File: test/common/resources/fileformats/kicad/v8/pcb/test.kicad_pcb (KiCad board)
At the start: 2 copper layers, 4 parts

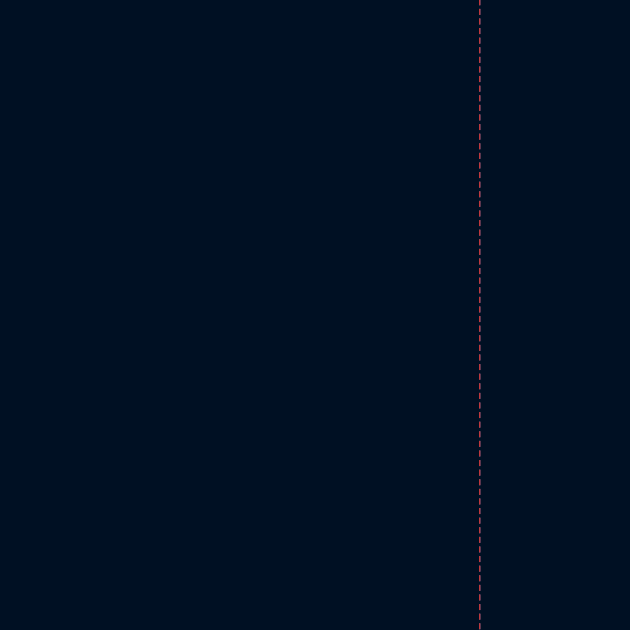
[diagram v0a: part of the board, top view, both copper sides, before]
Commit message: reset test file
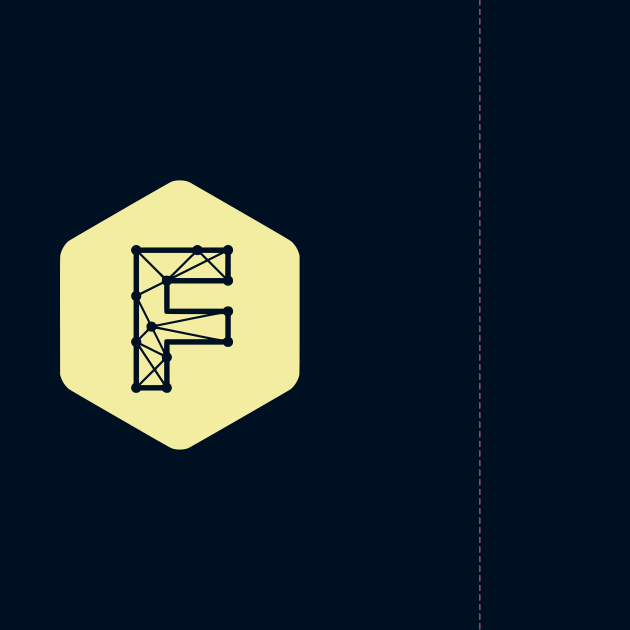
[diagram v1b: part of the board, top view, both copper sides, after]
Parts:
- G***: moved to F.Cu
- moved G*** 22.4 mm to (10.0, 20.0), turned to 0 degrees

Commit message: fast without cacheing
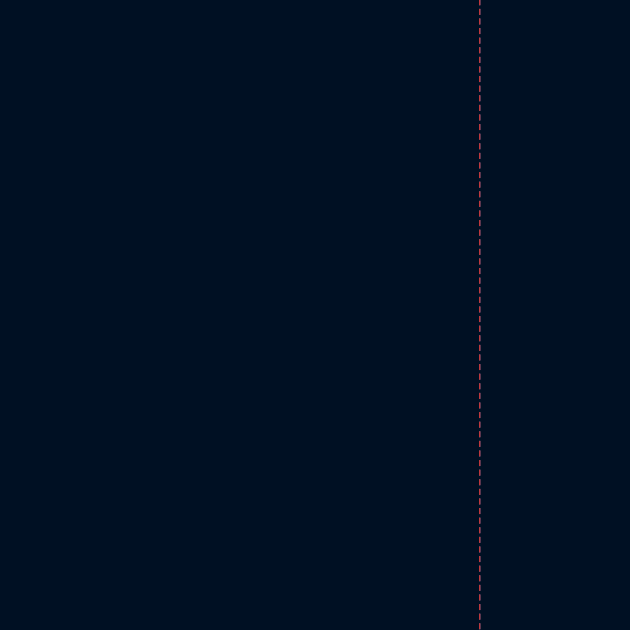
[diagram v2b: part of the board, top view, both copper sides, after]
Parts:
- G***: moved to B.Cu
- turned G*** to 90 degrees
